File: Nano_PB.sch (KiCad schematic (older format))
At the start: 0 parts

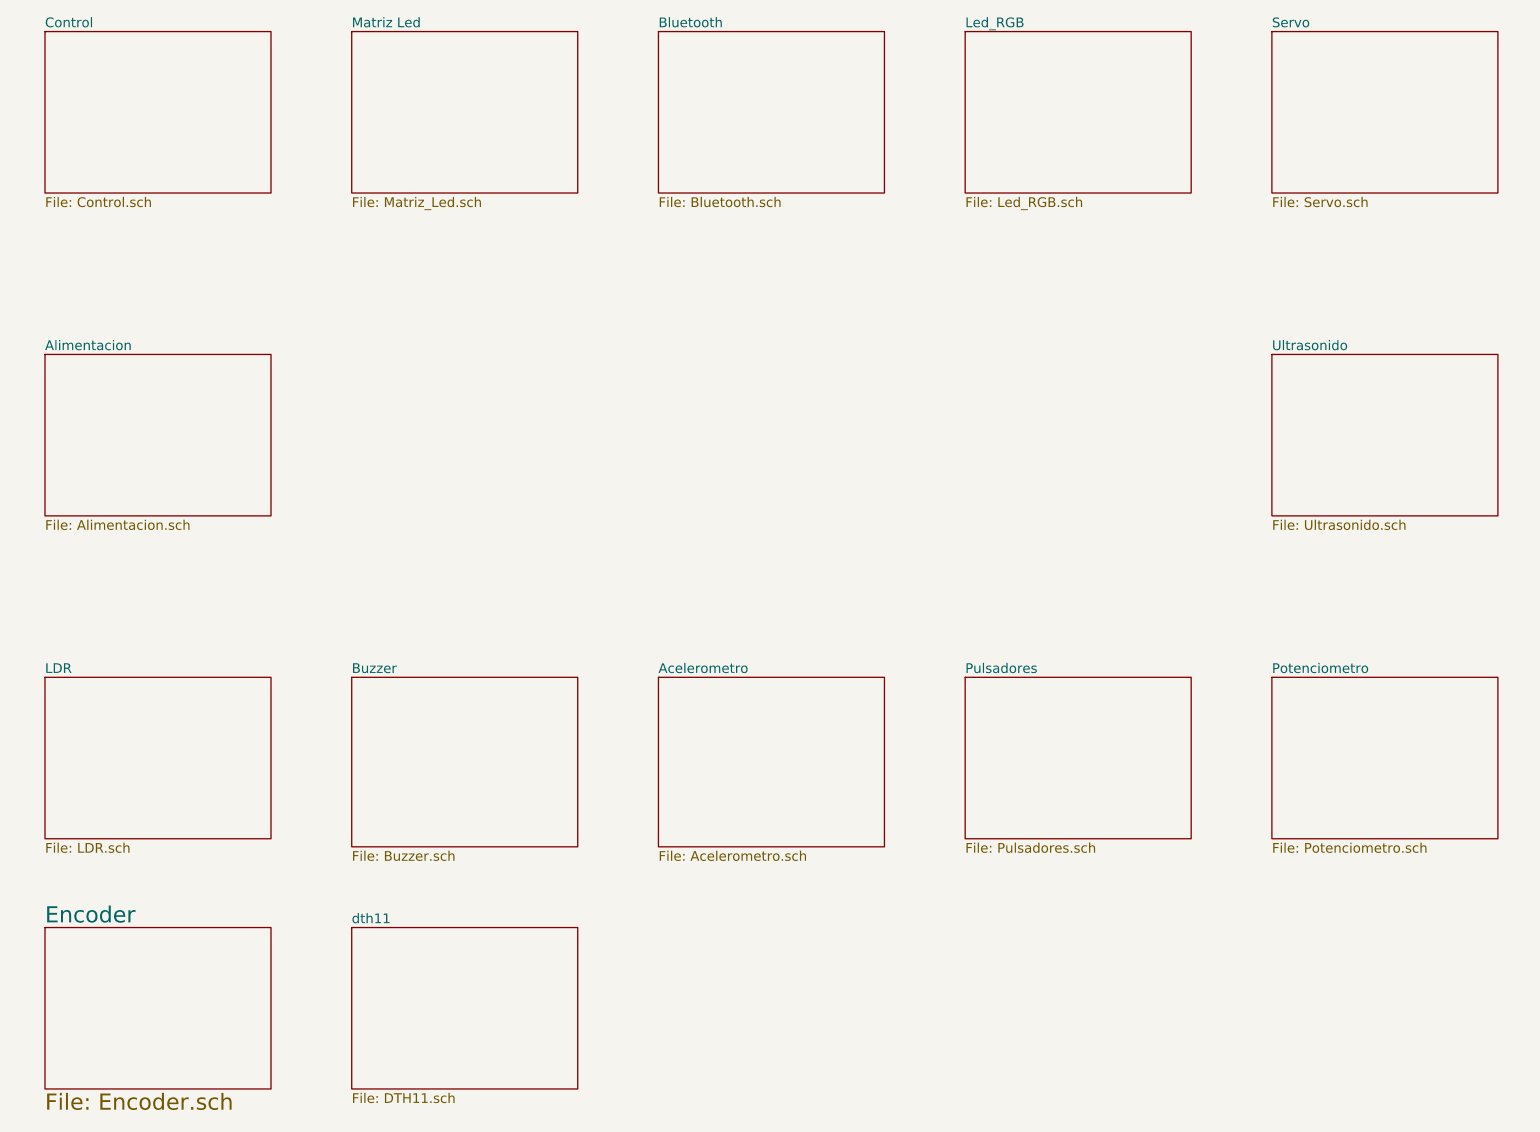
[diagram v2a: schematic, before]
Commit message: Actualizado el esquema electrico
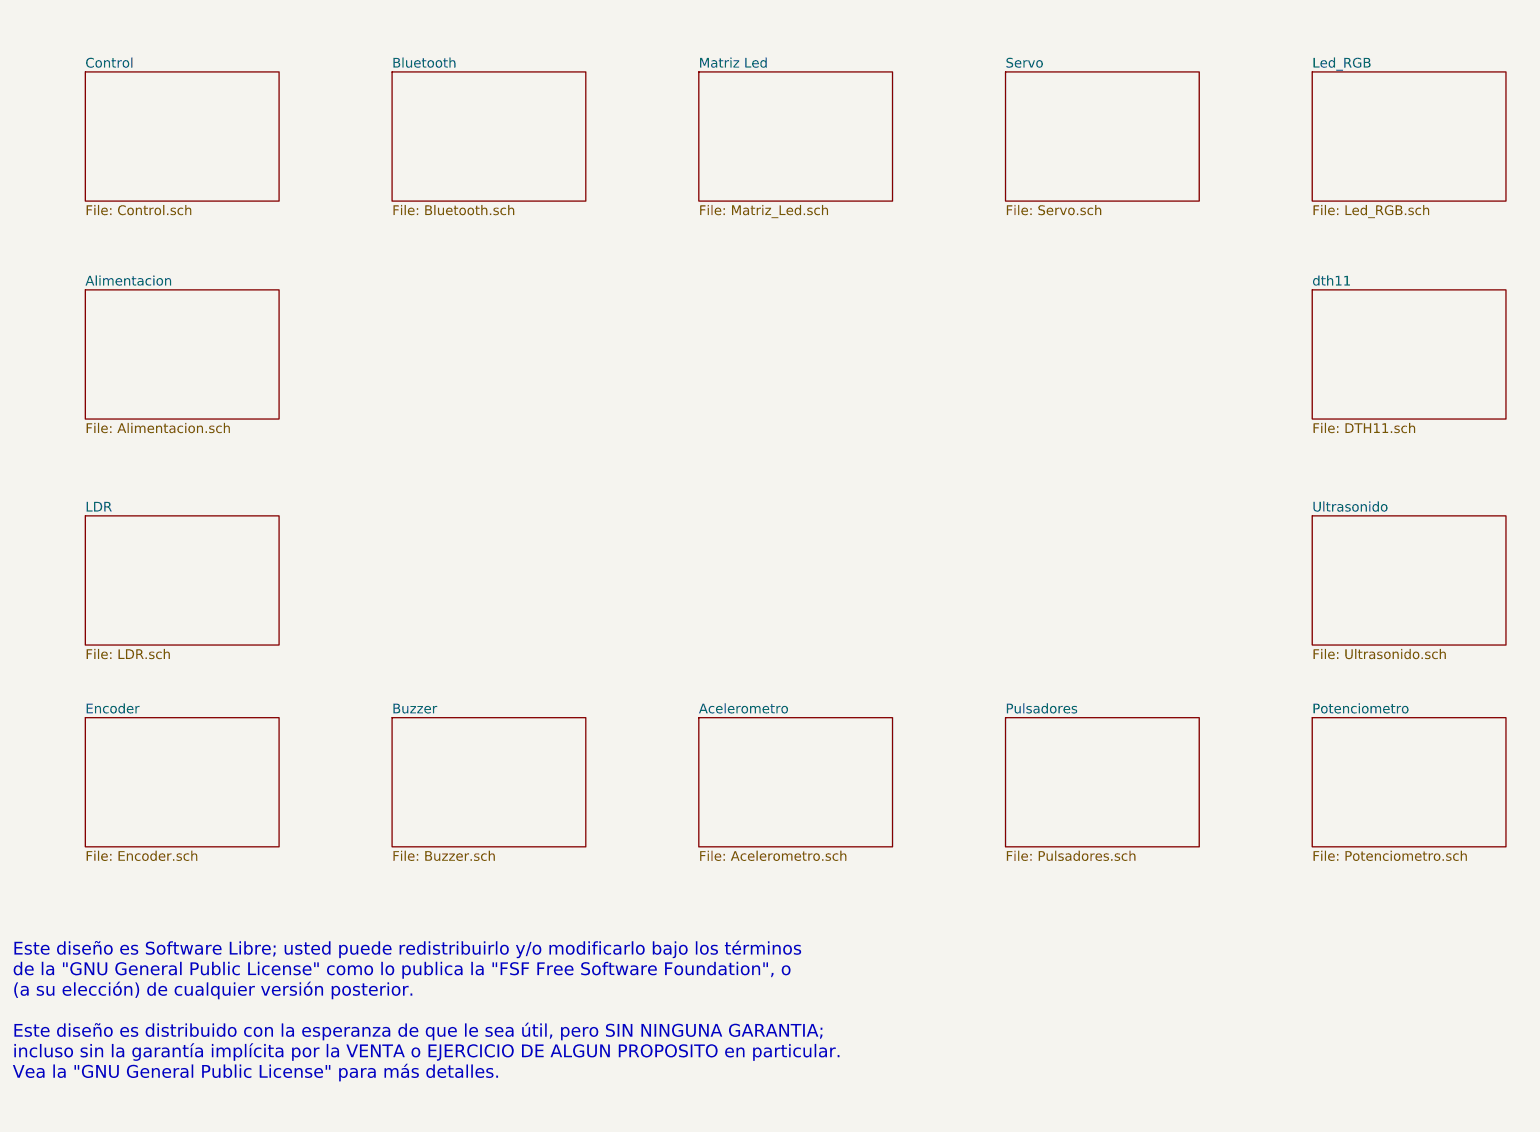
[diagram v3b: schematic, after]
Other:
- note added: "Este diseño es Software Libre; usted puede redistribuirlo y/o modificarlo bajo los términos\nde la "GNU General Public License" como lo publica la "FSF Free Software Foundation", o \n(a su elección) de cualquier versión posterior.\n\nEste diseño es distribuido con la esperanza de que le sea útil, pero SIN NINGUNA GARANTIA; \nincluso sin la garantía implícita por la VENTA o EJERCICIO DE ALGUN PROP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"
